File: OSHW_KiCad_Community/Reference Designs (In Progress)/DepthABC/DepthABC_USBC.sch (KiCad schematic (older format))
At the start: 59 parts, among them J13 DF23C-50DP-0.5V_92_, J5 USBC 3.1 Vertical, U1 2-bit bidirectional level shi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, U6 USB Type-C Switch, U7 USB Type-C Port Control

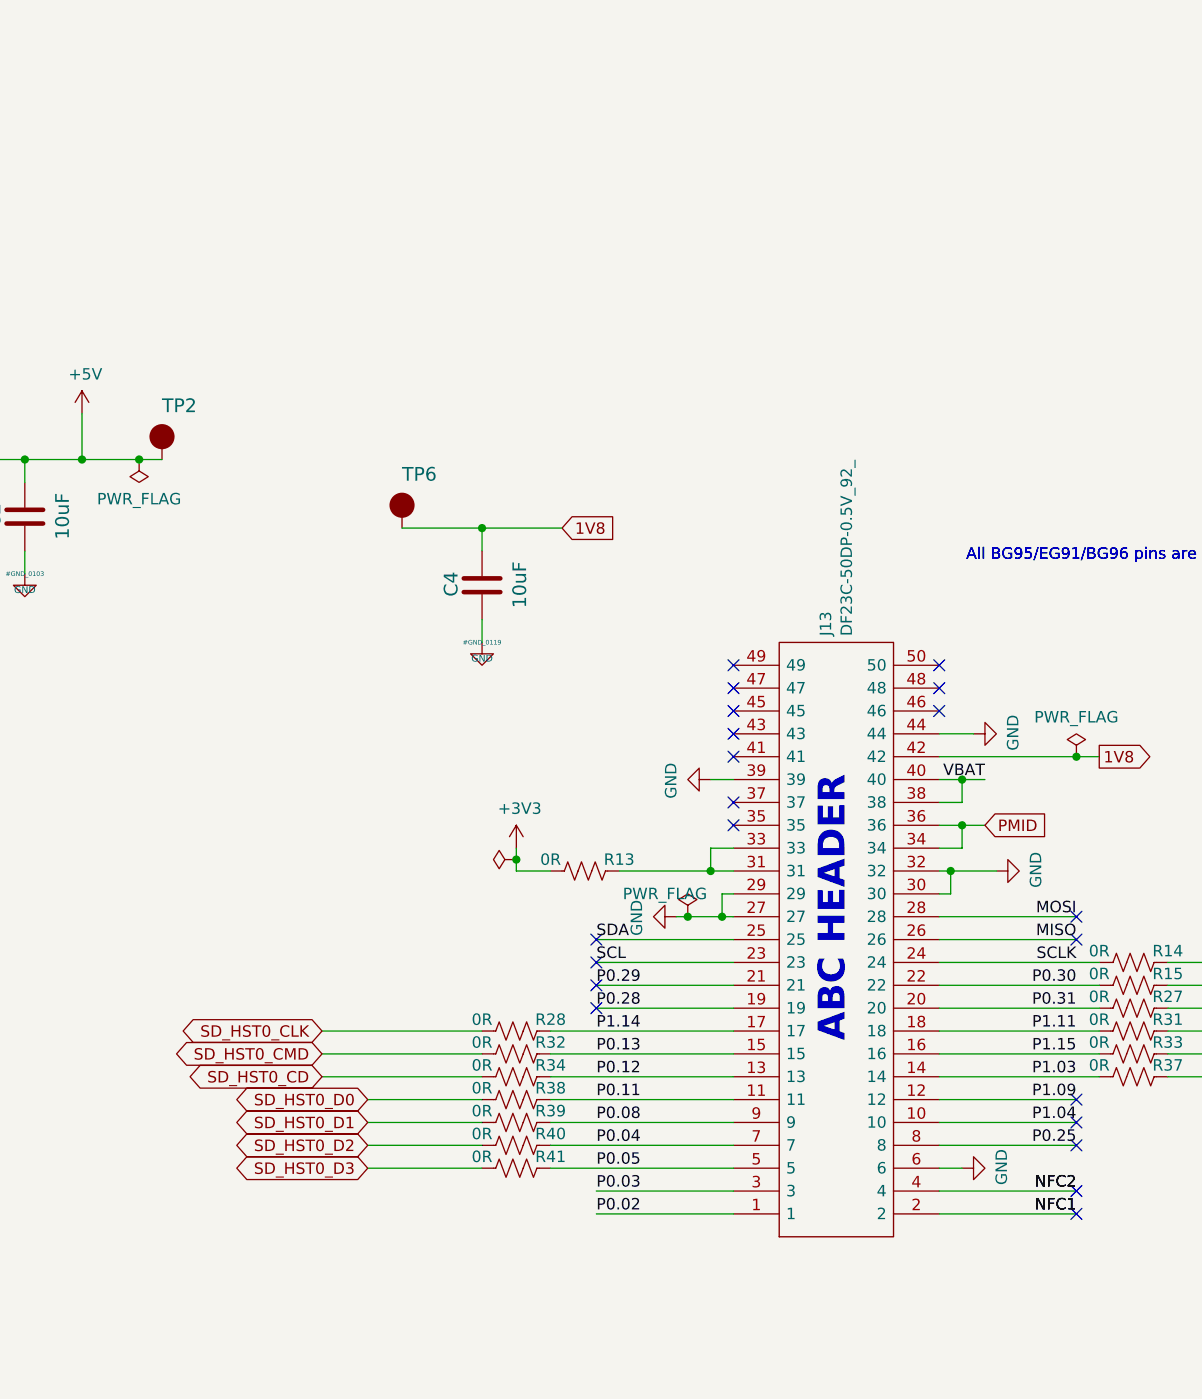
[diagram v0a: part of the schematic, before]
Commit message: abc final stages
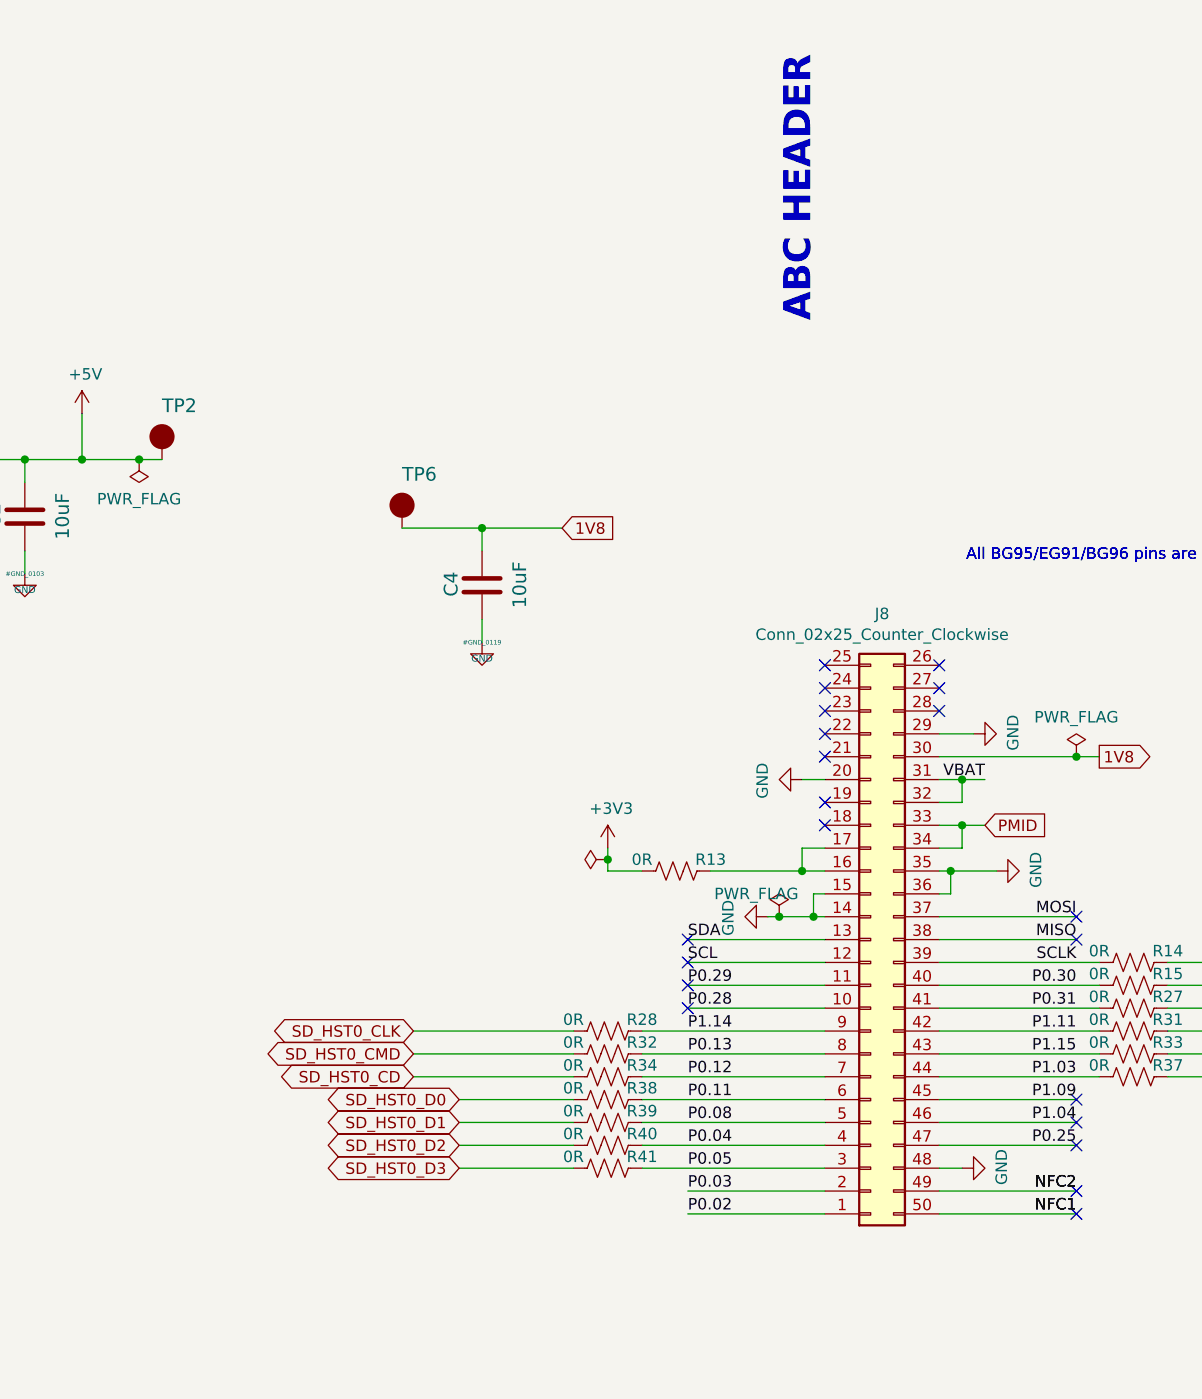
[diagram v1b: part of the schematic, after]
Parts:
- removed J13: DF23C-50DP-0.5V_92_, ABC:DF23C-50DS-0.5V(51), symbol DepthABC-rescue:SamacSys_Parts_DF23C-50DP-0.5V_92_-ABCDCBA-cache-BW1098ABC-resc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
- added J8: Conn_02x25_Counter_Clockwise, ABC:DF23C-50DS-0.5V(51), symbol Connector_Generic:Conn_02x25_Counter_Clockwise
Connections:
- net 1V8: now also J8.30 (Pin_30)
- net GND: now also J8.14 (Pin_14), J8.15 (Pin_15), J8.20 (Pin_20), J8.29 (Pin_29), J8.35 (Pin_35), J8.36 (Pin_36), J8.48 (Pin_48)
- net MISO: now also J8.38 (Pin_38)
- net MOSI: now also J8.37 (Pin_37)
- net NFC1: now also J8.50 (Pin_50)
- net NFC2: now also J8.49 (Pin_49)
- net P0.02: now also J8.1 (Pin_1)
- net P0.03: now also J8.2 (Pin_2)
- net P0.04: now also J8.4 (Pin_4)
- net P0.05: now also J8.3 (Pin_3)
- net P0.08: now also J8.5 (Pin_5)
- net P0.11: now also J8.6 (Pin_6)
- net P0.12: now also J8.7 (Pin_7)
- net P0.13: now also J8.8 (Pin_8)
- net P0.25: now also J8.47 (Pin_47)
- net P0.28: now also J8.10 (Pin_10)
- net P0.29: now also J8.11 (Pin_11)
- net P0.30: now also J8.40 (Pin_40)
- net P0.31: now also J8.41 (Pin_41)
- net P1.03: now also J8.44 (Pin_44)
- net P1.04: now also J8.46 (Pin_46)
- net P1.09: now also J8.45 (Pin_45)
- net P1.11: now also J8.42 (Pin_42)
- net P1.14: now also J8.9 (Pin_9)
- net P1.15: now also J8.43 (Pin_43)
- net PMID: now also J8.33 (Pin_33), J8.34 (Pin_34)
- net SCL: now also J8.12 (Pin_12)
- net SCLK: now also J8.39 (Pin_39)
- net SDA: now also J8.13 (Pin_13)
- net VBAT: now also J8.31 (Pin_31), J8.32 (Pin_32)
- net at R13.1: now also J8.16 (Pin_16), J8.17 (Pin_17)
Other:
- moved on the sheet: R13, R28, R32, R34, R38, R39, R40, R41

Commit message: fab changes to abc
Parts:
- C1, C2, C32, C33, C34, C35, C36, C37, C38, C39, C4: Population (none) -> Y; Substitutes  (none) -> Y
- H10, H11, H12, H9: Short Description (none) -> ABC mount
- J5: MPN1 (none) -> 10132328-10011LF; Population (none) -> Y; STANDARD Manufacturer Recommendations -> (none); Substitutes  (none) -> N
- J8: MANUFACTURER (none) -> Amphenol; MPN1 (none) -> DF23C-50DS-0.5V(51); Population (none) -> Y; Short Description (none) -> ABC header; Substitutes  (none) -> N
- MISC2: MANUFACTURER (none) -> Luxonis
- R11, R12, R13, R14, R15, R16, R17, R18, R19, R20, R21, R22, R23, R24, R25, R26, R27, R28, R31, R32, R33, R34, R37, R38, R39, R40, R41, R5, R6, R7: Population (none) -> Y; STANDARD 1/10W 1% -> 1%; Substitutes  (none) -> Y; Voltage Rating (none) -> 1/10W
- U1, U6: MANUFACTURER (none) -> TI; Population (none) -> Y; Substitutes  (none) -> N
- U7: footprint Luxonis_KiCad_Master:Texas_Instruments-RWB0012A-0-0-MFG -> Luxonis_KiCad_Master:Texas_Instruments-TUSB321RWBR; MANUFACTURER (none) -> TI; Population (none) -> Y; Substitutes  (none) -> N
